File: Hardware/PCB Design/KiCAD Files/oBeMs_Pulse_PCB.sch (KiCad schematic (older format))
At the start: 16 parts, among them P1 1WIRE, P3 HARD_WDT, P4 LED 5-8, P5 AC_INPUT_PLUG, P6 AC_INPUT, P7 LED 1-4, P8 LT_PWR

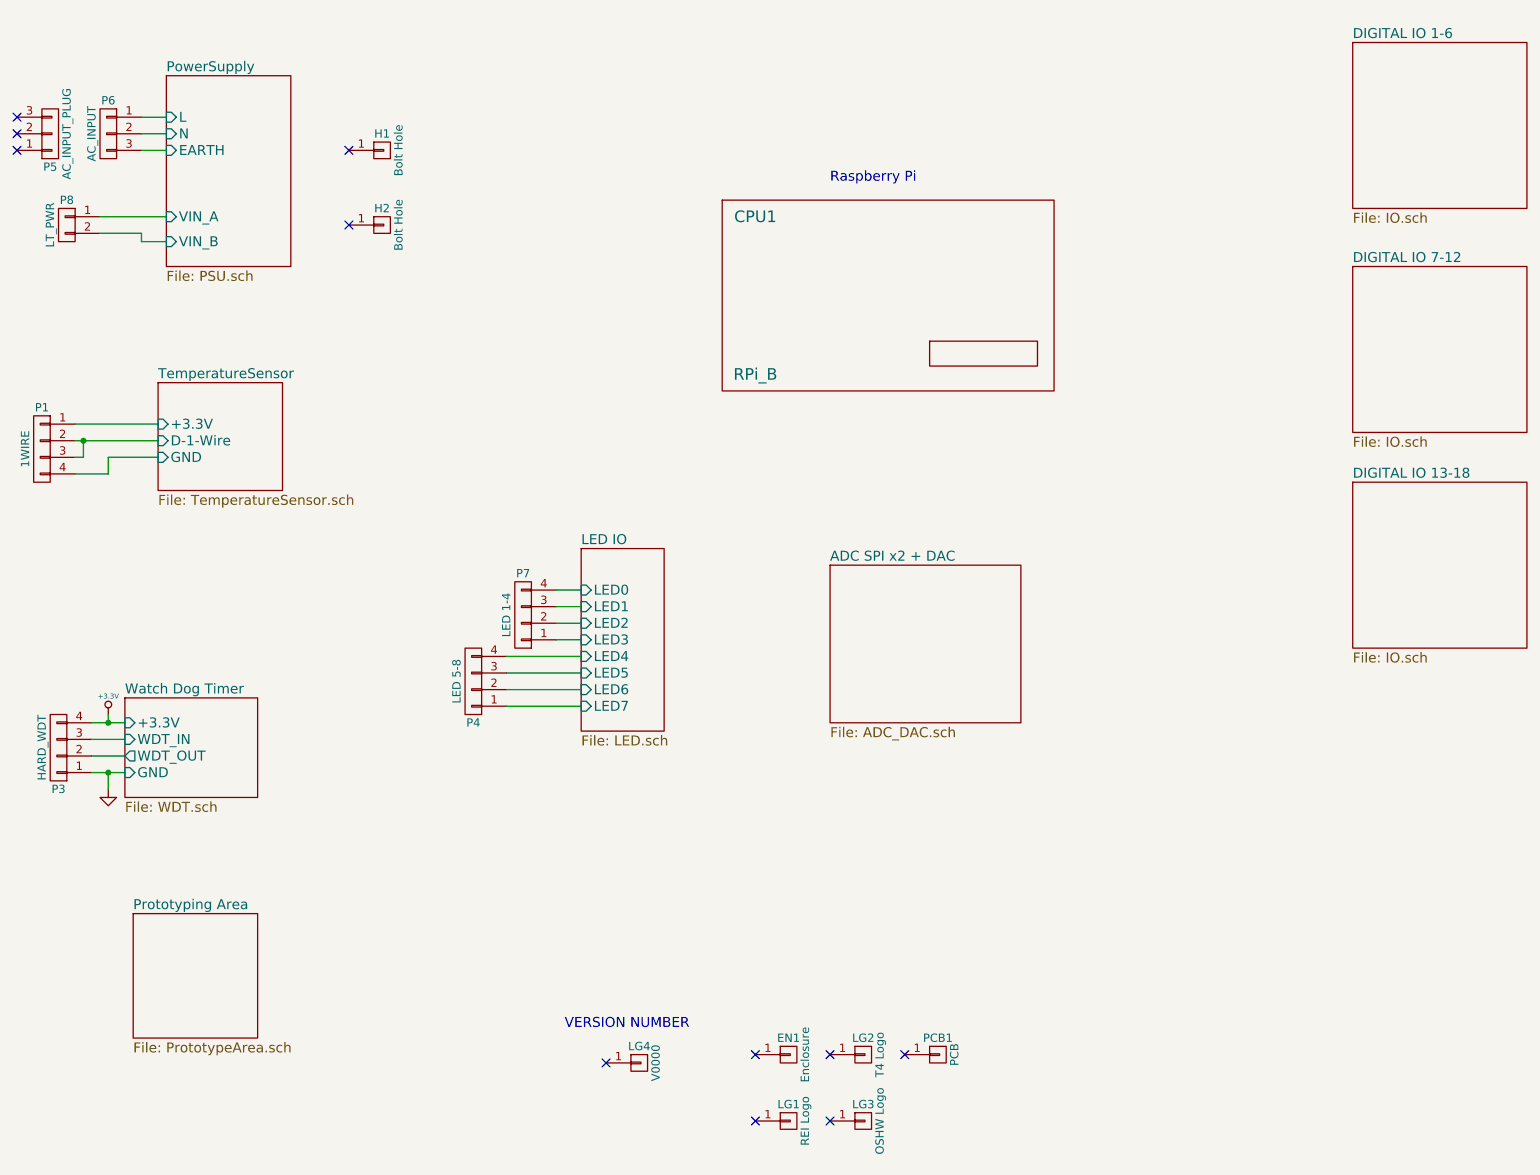
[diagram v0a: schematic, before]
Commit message: Rev 6. Final changes before PCB v0000 done
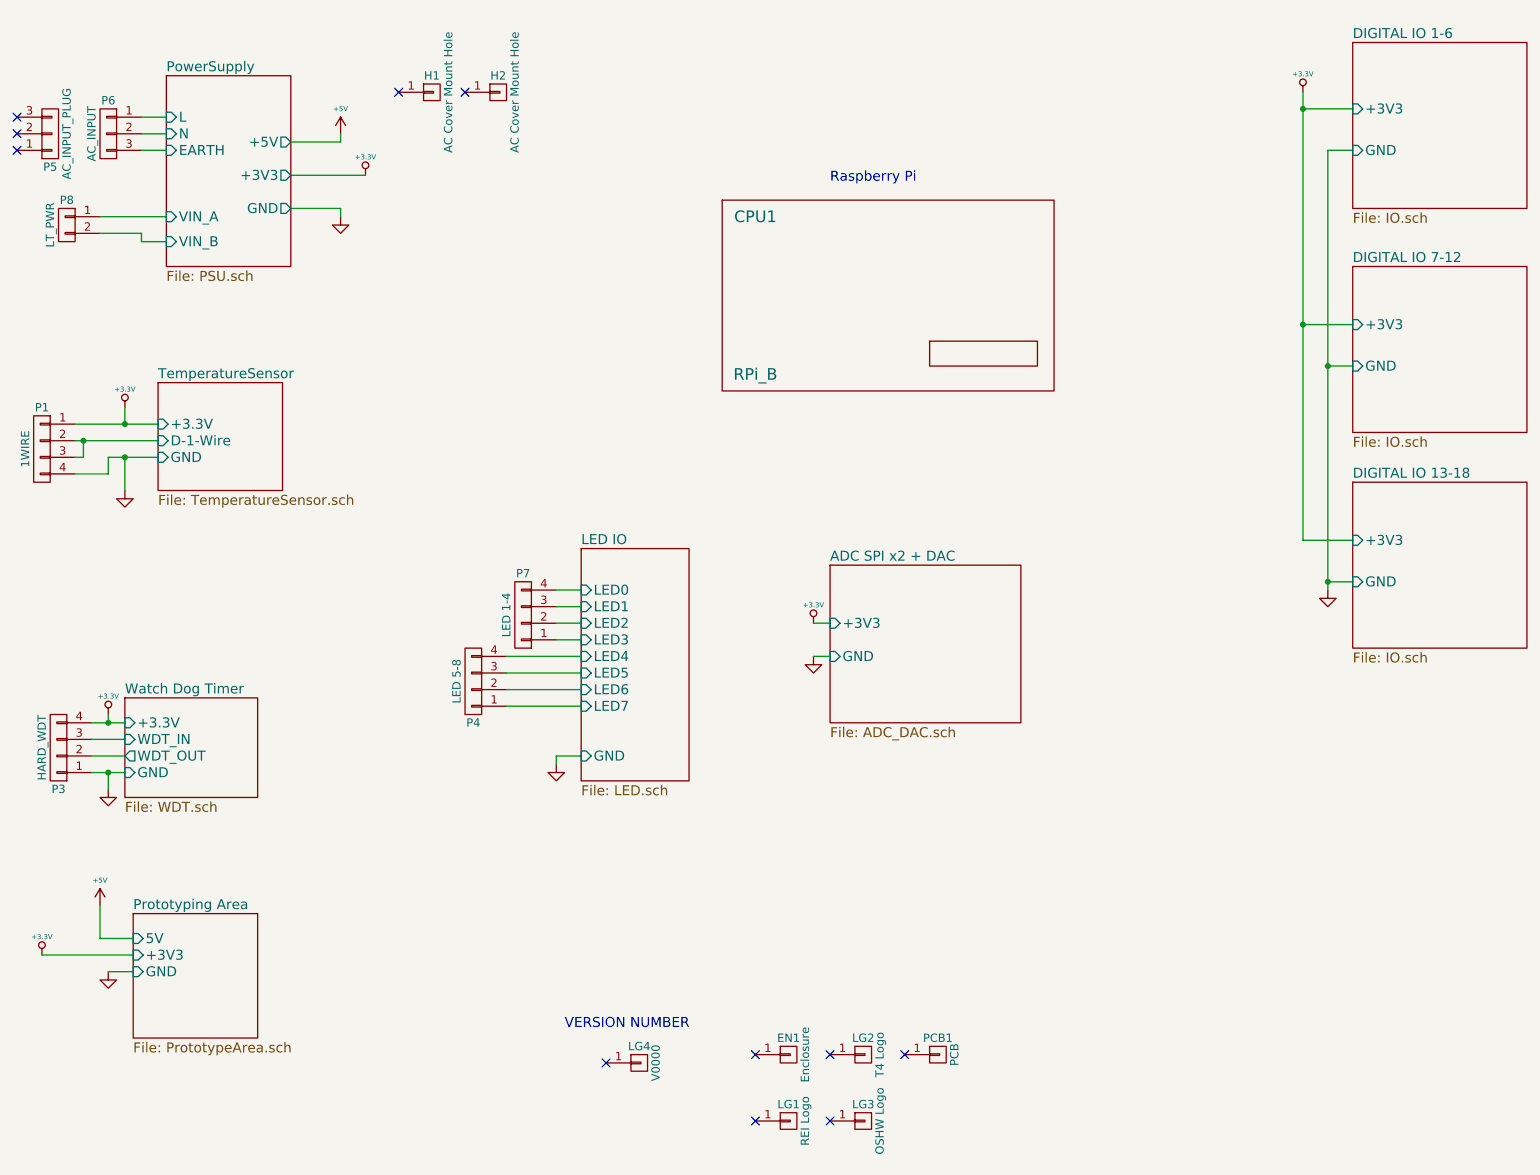
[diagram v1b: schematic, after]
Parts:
- H1, H2: value Bolt Hole -> AC Cover Mount Hole
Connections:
- net TemperatureSensor/+3.3V is gone; now on net +3.3V: P1.1 (P1)
- net TemperatureSensor/GND is gone; now on net GND: P1.4 (P4)
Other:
- moved on the sheet: H1, H2
